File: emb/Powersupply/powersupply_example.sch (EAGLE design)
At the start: 15 parts, among them IC1 7805TV, IC2 7812TV, IC3 LM2574N-5.0

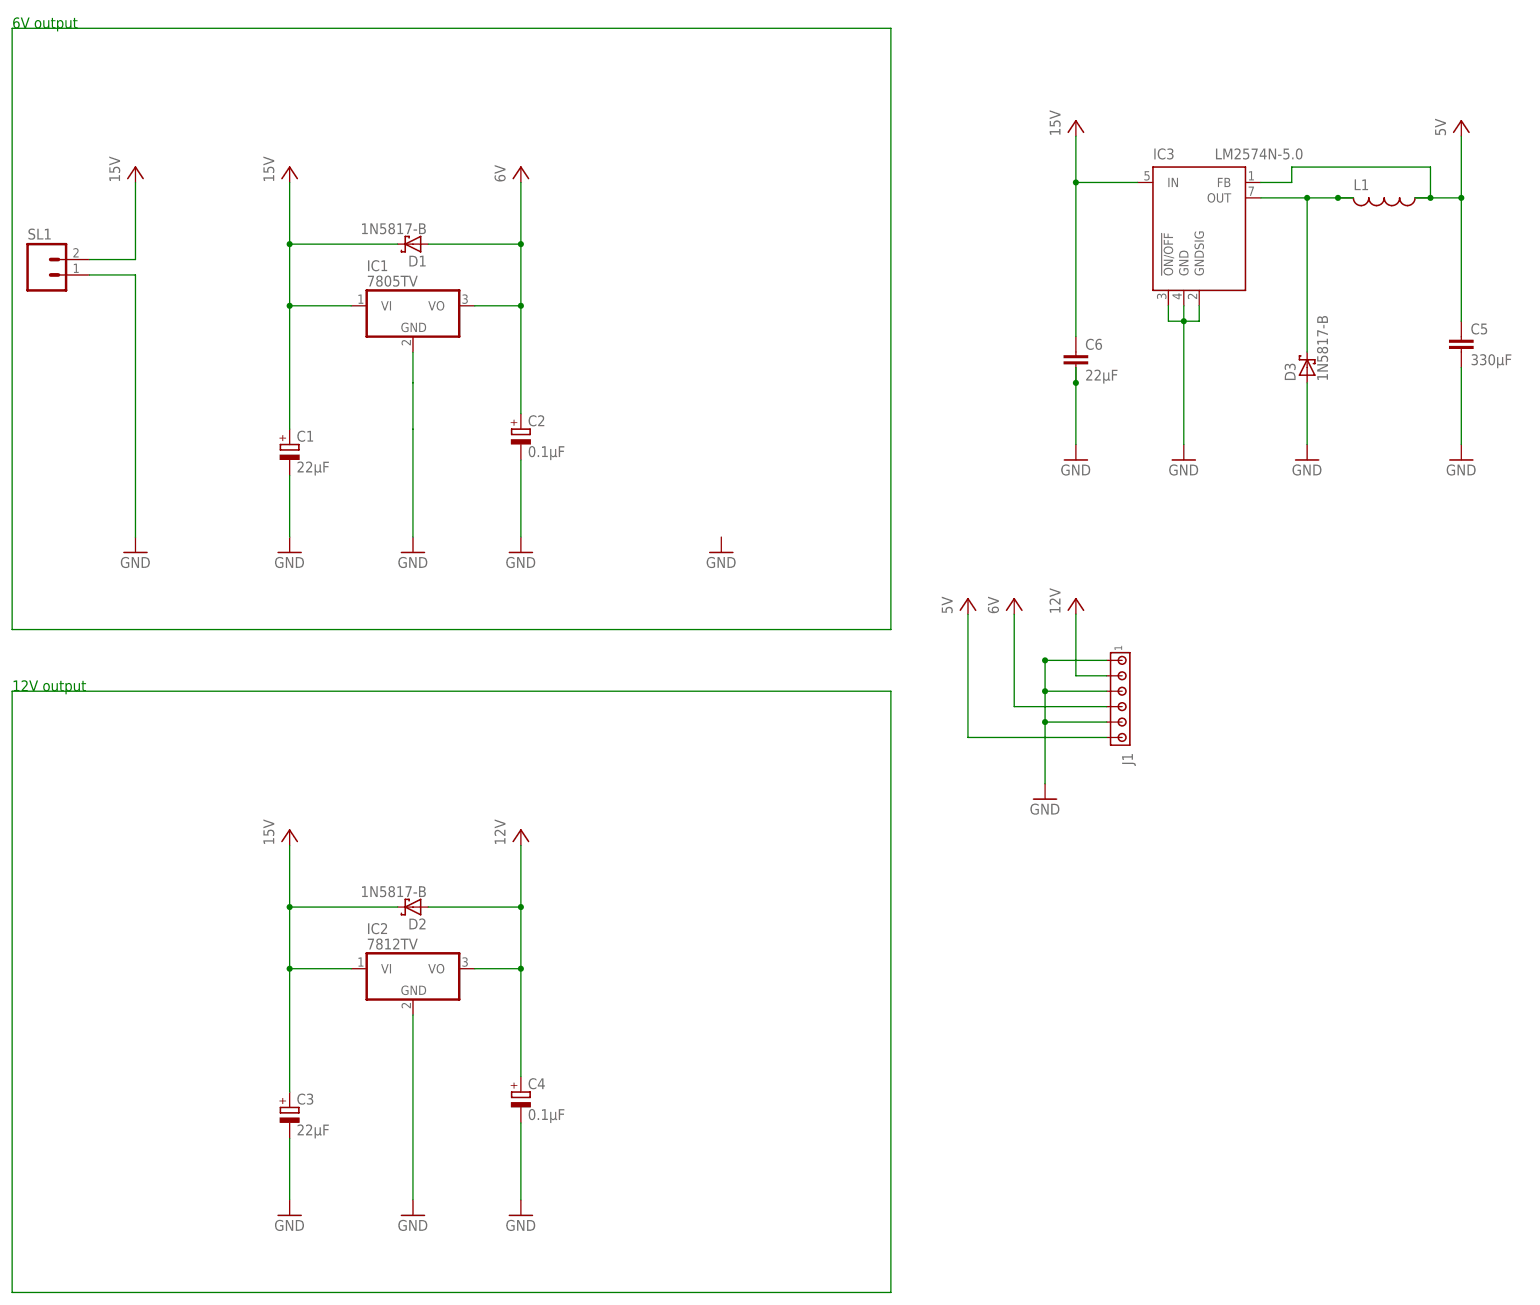
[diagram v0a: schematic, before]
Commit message: Updated PCB board
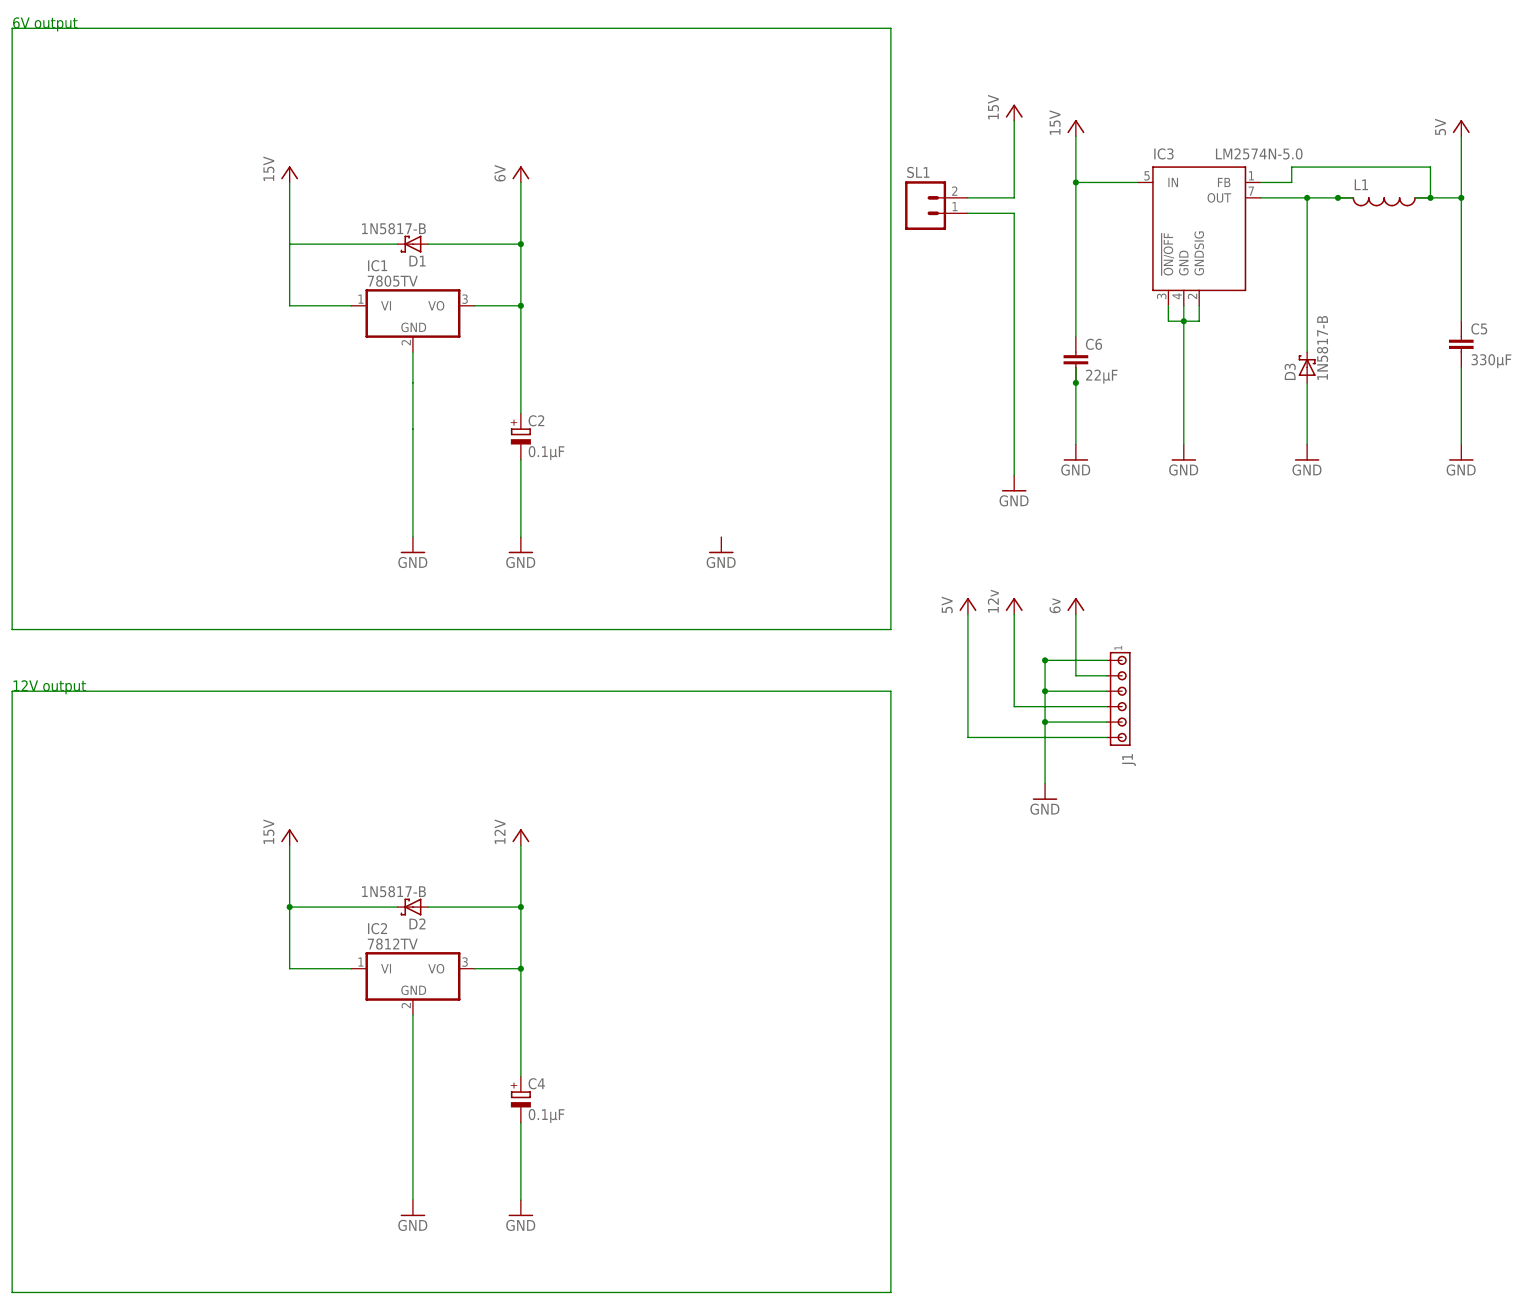
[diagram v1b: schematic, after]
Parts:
- removed C1, C3: 22µF, rcl:CPOL-EUE2.5-5
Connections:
- net 12V: now also J1.4; no longer J1.2
- net 15V: no longer C1.+, C3.+
- net 6V: now also J1.2; no longer J1.4
- net GND: no longer C1.-, C3.-
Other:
- moved on the sheet: SL1
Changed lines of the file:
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@@
 <part name="P+2" library="supply1" deviceset="VCC" device="" value="15V"/>
 <part name="P+3" library="supply1" deviceset="VCC" device="" value="6V"/>
-<part name="P+4" library="supply1" deviceset="VCC" device="" value="6V"/>
+<part name="P+4" library="supply1" deviceset="VCC" device="" value="12v"/>
 <part name="SL1" library="con-amp-quick" deviceset="M02" device=""/>
 <part name="GND1" library="supply1" deviceset="GND" device=""/>
-<part name="GND2" library="supply1" deviceset="GND" device=""/>
 <part name="GND3" library="supply1" deviceset="GND" device=""/>
 <part name="GND4" library="supply1" deviceset="GND" device=""/>
 <part name="GND5" library="supply1" deviceset="GND" device=""/>
-<part name="C1" library="rcl" deviceset="CPOL-EU" device="E2.5-5" value="22µF"/>
 <part name="C2" library="rcl" deviceset="CPOL-EU" device="E2.5-5" value="0.1µF"/>
 <part name="D1" library="diode" deviceset="1N581*" device="" technology="7-B"/>
@@
 <part name="P+5" library="supply1" deviceset="VCC" device="" value="12V"/>
 <part name="P+6" library="supply1" deviceset="VCC" device="" value="5V"/>
-<part name="GND7" library="supply1" deviceset="GND" device=""/>
 <part name="GND8" library="supply1" deviceset="GND" device=""/>
 <part name="GND9" library="supply1" deviceset="GND" device=""/>
 <part name="GND10" library="supply1" deviceset="GND" device=""/>
-<part name="C3" library="rcl" deviceset="CPOL-EU" device="E2.5-5" value="22µF"/>
 <part name="C4" library="rcl" deviceset="CPOL-EU" device="E2.5-5" value="0.1µF"/>
 <part name="D2" library="diode" deviceset="1N581*" device="" technology="7-B"/>
@@
 <part name="GND12" library="supply1" deviceset="GND" device=""/>
 <part name="GND13" library="supply1" deviceset="GND" device=""/>
-<part name="P+8" library="supply1" deviceset="VCC" device="" value="12V"/>
+<part name="P+8" library="supply1" deviceset="VCC" device="" value="6v"/>
 <part name="5V" library="supply1" deviceset="VCC" device="" value="5V"/>
 <part name="L1" library="resistor" deviceset="L-US" device="0204/7"/>
@@
 </plain>
 <instances>
-<instance part="15V" gate="VCC" x="-33.02" y="88.9"/>
+<instance part="15V" gate="VCC" x="111.76" y="99.06"/>
 <instance part="P+2" gate="VCC" x="-7.62" y="88.9"/>
 <instance part="P+3" gate="VCC" x="30.48" y="88.9"/>
 <instance part="P+4" gate="VCC" x="111.76" y="17.78"/>
-<instance part="SL1" gate="G$1" x="-48.26" y="71.12"/>
-<instance part="GND1" gate="1" x="-33.02" y="25.4"/>
-<instance part="GND2" gate="1" x="-7.62" y="25.4"/>
+<instance part="SL1" gate="G$1" x="96.52" y="81.28"/>
+<instance part="GND1" gate="1" x="111.76" y="35.56"/>
 <instance part="GND3" gate="1" x="30.48" y="25.4"/>
 <instance part="GND4" gate="1" x="12.7" y="25.4"/>
 <instance part="GND5" gate="1" x="63.5" y="25.4"/>
-<instance part="C1" gate="G$1" x="-7.62" y="43.18"/>
 <instance part="C2" gate="G$1" x="30.48" y="45.72"/>
 <instance part="D1" gate="G$1" x="12.7" y="76.2" rot="R180"/>
@@
 <instance part="P+5" gate="VCC" x="30.48" y="-20.32"/>
 <instance part="P+6" gate="VCC" x="104.14" y="17.78"/>
-<instance part="GND7" gate="1" x="-7.62" y="-83.82"/>
 <instance part="GND8" gate="1" x="30.48" y="-83.82"/>
 <instance part="GND9" gate="1" x="12.7" y="-83.82"/>
 <instance part="GND10" gate="1" x="116.84" y="-15.24"/>
-<instance part="C3" gate="G$1" x="-7.62" y="-66.04"/>
 <instance part="C4" gate="G$1" x="30.48" y="-63.5"/>
 <instance part="D2" gate="G$1" x="12.7" y="-33.02" rot="R180"/>
@@
 <pinref part="GND1" gate="1" pin="GND"/>
 <pinref part="SL1" gate="G$1" pin="1"/>
-<wire x1="-33.02" y1="27.94" x2="-33.02" y2="71.12" width="0.1524" layer="91"/>
-<wire x1="-33.02" y1="71.12" x2="-40.64" y2="71.12" width="0.1524" layer="91"/>
+<wire x1="111.76" y1="38.1" x2="111.76" y2="81.28" width="0.1524" layer="91"/>
+<wire x1="111.76" y1="81.28" x2="104.14" y2="81.28" width="0.1524" layer="91"/>
 </segment>
 <segment>
@@
 </segment>
 <segment>
-<pinref part="C1" gate="G$1" pin="-"/>
-<pinref part="GND2" gate="1" pin="GND"/>
-<wire x1="-7.62" y1="38.1" x2="-7.62" y2="27.94" width="0.1524" layer="91"/>
-</segment>
-<segment>
 <pinref part="C2" gate="G$1" pin="-"/>
 <pinref part="GND3" gate="1" pin="GND"/>
@@
 <wire x1="12.7" y1="-81.28" x2="12.7" y2="-50.8" width="0.1524" layer="91"/>
 <pinref part="IC2" gate="A1" pin="GND"/>
-</segment>
-<segment>
-<pinref part="C3" gate="G$1" pin="-"/>
-<pinref part="GND7" gate="1" pin="GND"/>
-<wire x1="-7.62" y1="-71.12" x2="-7.62" y2="-81.28" width="0.1524" layer="91"/>
 </segment>
 <segment>
@@
 <pinref part="15V" gate="VCC" pin="VCC"/>
 <pinref part="SL1" gate="G$1" pin="2"/>
-<wire x1="-33.02" y1="86.36" x2="-33.02" y2="73.66" width="0.1524" layer="91"/>
-<wire x1="-33.02" y1="73.66" x2="-40.64" y2="73.66" width="0.1524" layer="91"/>
-</segment>
-<segment>
-<pinref part="P+2" gate="VCC" pin="VCC"/>
-<pinref part="C1" gate="G$1" pin="+"/>
-<wire x1="-7.62" y1="86.36" x2="-7.62" y2="76.2" width="0.1524" layer="91"/>
-<wire x1="-7.62" y1="76.2" x2="-7.62" y2="66.04" width="0.1524" layer="91"/>
-<wire x1="-7.62" y1="66.04" x2="-7.62" y2="45.72" width="0.1524" layer="91"/>
-<wire x1="10.16" y1="76.2" x2="-7.62" y2="76.2" width="0.1524" layer="91"/>
-<junction x="-7.62" y="76.2"/>
-<pinref part="D1" gate="G$1" pin="C"/>
-<pinref part="IC1" gate="A1" pin="VI"/>
-<wire x1="2.54" y1="66.04" x2="-7.62" y2="66.04" width="0.1524" layer="91"/>
-<junction x="-7.62" y="66.04"/>
+<wire x1="111.76" y1="96.52" x2="111.76" y2="83.82" width="0.1524" layer="91"/>
+<wire x1="111.76" y1="83.82" x2="104.14" y2="83.82" width="0.1524" layer="91"/>
 </segment>
 <segment>
 <pinref part="P+1" gate="VCC" pin="VCC"/>
-<pinref part="C3" gate="G$1" pin="+"/>
 <wire x1="-7.62" y1="-22.86" x2="-7.62" y2="-33.02" width="0.1524" layer="91"/>
 <wire x1="-7.62" y1="-33.02" x2="-7.62" y2="-43.18" width="0.1524" layer="91"/>
-<wire x1="-7.62" y1="-43.18" x2="-7.62" y2="-63.5" width="0.1524" layer="91"/>
 <wire x1="10.16" y1="-33.02" x2="-7.62" y2="-33.02" width="0.1524" layer="91"/>
 <junction x="-7.62" y="-33.02"/>
 <pinref part="D2" gate="G$1" pin="C"/>
 <wire x1="2.54" y1="-43.18" x2="-7.62" y2="-43.18" width="0.1524" layer="91"/>
-<junction x="-7.62" y="-43.18"/>
 <pinref part="IC2" gate="A1" pin="VI"/>
 </segment>
@@
 <wire x1="121.92" y1="60.96" x2="121.92" y2="86.36" width="0.1524" layer="91"/>
 <junction x="121.92" y="86.36"/>
+</segment>
+<segment>
+<pinref part="P+2" gate="VCC" pin="VCC"/>
+<wire x1="-7.62" y1="86.36" x2="-7.62" y2="76.2" width="0.1524" layer="91"/>
+<pinref part="D1" gate="G$1" pin="C"/>
+<wire x1="10.16" y1="76.2" x2="-7.62" y2="76.2" width="0.1524" layer="91"/>
+<pinref part="IC1" gate="A1" pin="VI"/>
+<wire x1="2.54" y1="66.04" x2="-7.62" y2="66.04" width="0.1524" layer="91"/>
+<wire x1="-7.62" y1="76.2" x2="-7.62" y2="66.04" width="0.1524" layer="91"/>
 </segment>
 </net>
@@
 </segment>
 <segment>
-<pinref part="P+4" gate="VCC" pin="VCC"/>
-<pinref part="J1" gate="G$1" pin="4"/>
-<wire x1="111.76" y1="15.24" x2="111.76" y2="0" width="0.1524" layer="91"/>
-<wire x1="111.76" y1="0" x2="127" y2="0" width="0.1524" layer="91"/>
+<pinref part="P+8" gate="VCC" pin="VCC"/>
+<pinref part="J1" gate="G$1" pin="2"/>
+<wire x1="121.92" y1="15.24" x2="121.92" y2="5.08" width="0.1524" layer="91"/>
+<wire x1="121.92" y1="5.08" x2="127" y2="5.08" width="0.1524" layer="91"/>
 </segment>
 </net>
@@
 </segment>
 <segment>
-<pinref part="P+8" gate="VCC" pin="VCC"/>
-<pinref part="J1" gate="G$1" pin="2"/>
-<wire x1="121.92" y1="15.24" x2="121.92" y2="5.08" width="0.1524" layer="91"/>
-<wire x1="121.92" y1="5.08" x2="127" y2="5.08" width="0.1524" layer="91"/>
-</segment>
-</net>
+<pinref part="P+4" gate="VCC" pin="VCC"/>
+<pinref part="J1" gate="G$1" pin="4"/>
+<wire x1="111.76" y1="15.24" x2="111.76" y2="0" width="0.1524" layer="91"/>
+<wire x1="111.76" y1="0" x2="127" y2="0" width="0.1524" layer="91"/>
+</segment>
+</net>
